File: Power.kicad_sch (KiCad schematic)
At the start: 56 parts, among them J7 MX1.25 2P, Q1 SI2305, Q2 SI2305, U1 SF32LB527UD6, U10 MT9700, U3 MT9700, U4 TPS563201, U5 ME6211C33M5, U7 MT3608

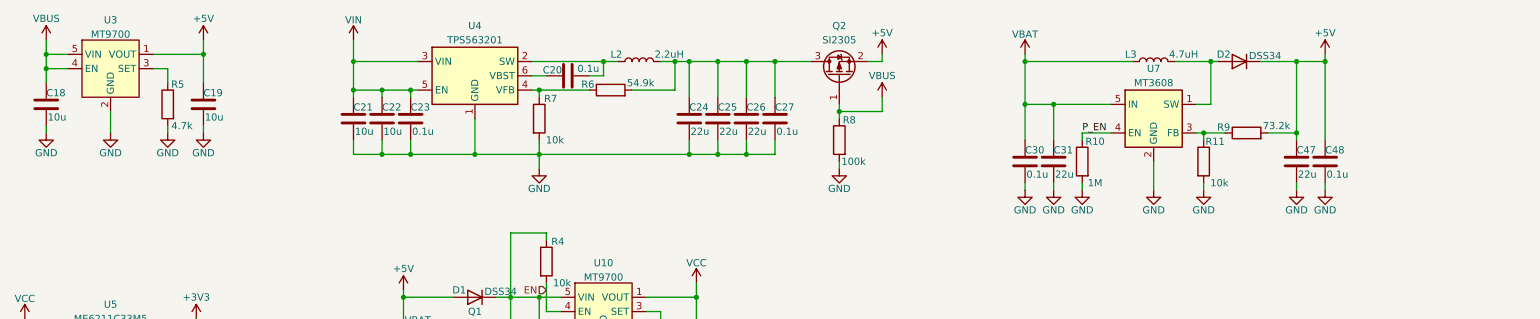
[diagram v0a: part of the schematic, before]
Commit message: fix: 修复电源架构
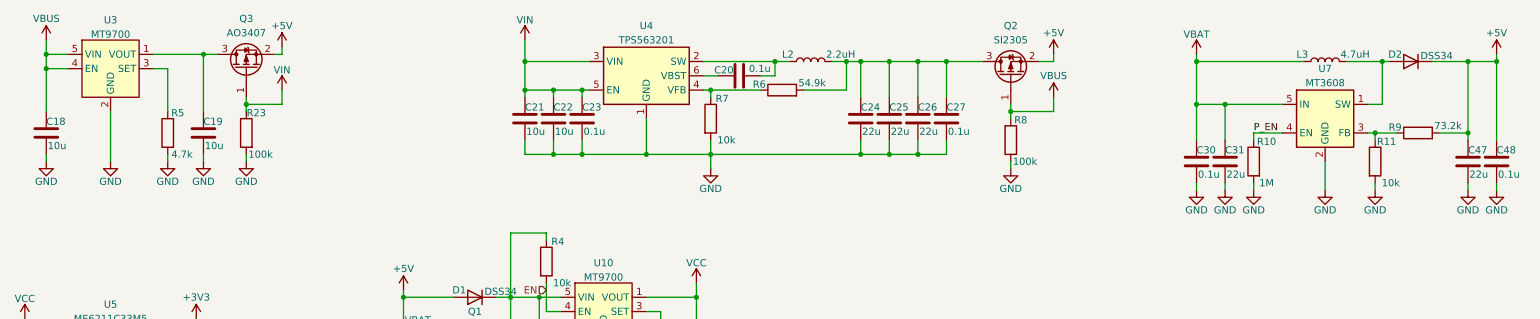
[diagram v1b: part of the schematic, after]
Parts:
- added Q3: AO3407, Package_TO_SOT_SMD:SOT-23, symbol Transistor_FET:AO3401A
- added R23: 100k, Resistor_SMD:R_0402_1005Metric, symbol Device:R
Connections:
- net +5V: now also Q3.2 (S); no longer C19.1, U3.1 (VOUT)
- net GND: now also R23.2
- net VIN: now also Q3.1 (G), R23.1
- new net: C19.1, Q3.3 (D), U3.1 (VOUT)
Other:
- moved on the sheet: C18, C19, C20, C21, C22, C23, C24, C25, C26, C27, C30, C31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
